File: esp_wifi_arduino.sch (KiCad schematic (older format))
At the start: 32 parts, among them IC1 ATMEGA328P-A, P1 CONN_01X15, P2 CONN_01X15, P5 CONN_01X04, P6 CONN_01X04, SW1 SW_PUSH, SW2 SW_PUSH, SW3 DIPSW4, U1 ADG3304, U2 ESP-WROOM-02, U3 NJM2391DL1-33, X1 16MHz

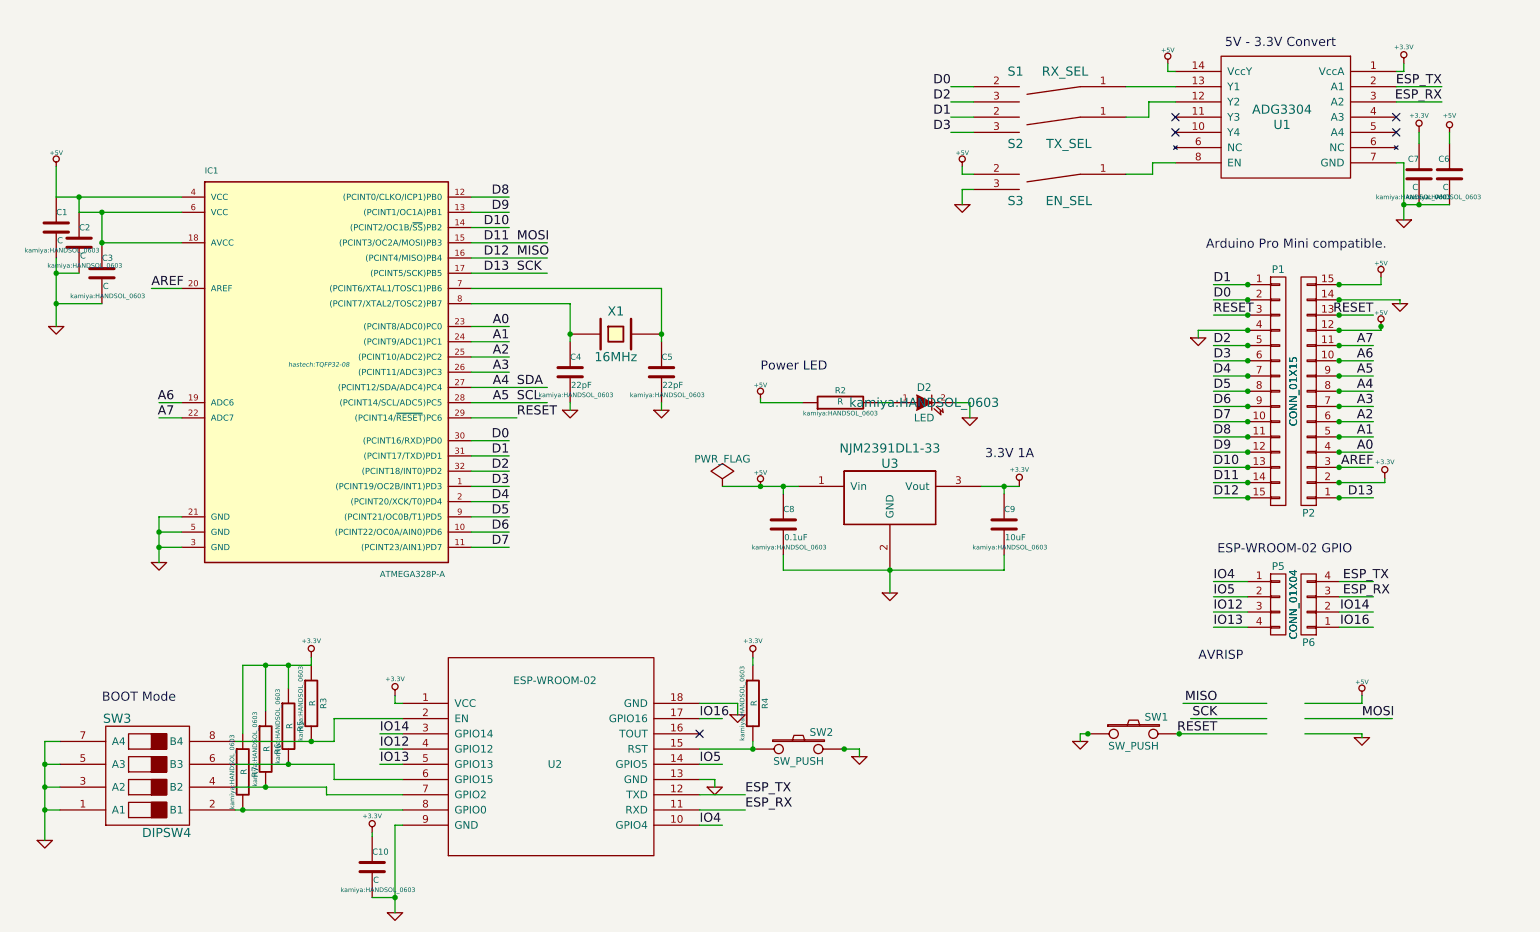
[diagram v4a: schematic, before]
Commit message: Draw Pattern
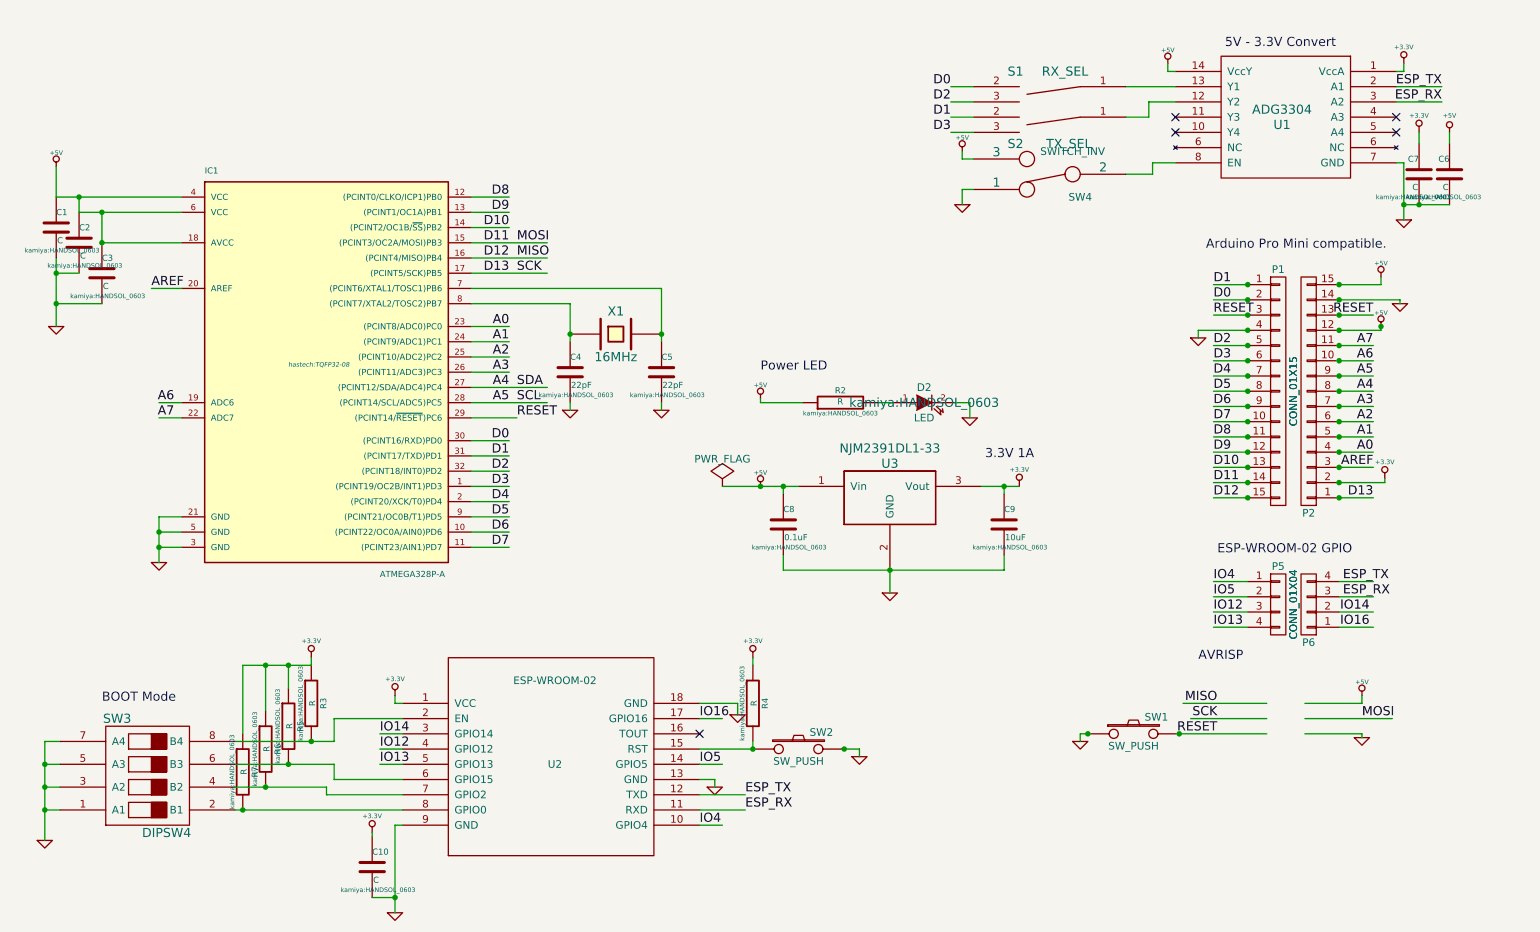
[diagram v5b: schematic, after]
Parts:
- removed S3: EN_SEL, kamiya:ALPS_SSSS213202(SlideSW), symbol SEL
- added SW4: SWITCH_INV, ~, symbol SWITCH_INV
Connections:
- wire segments 202 -> 178
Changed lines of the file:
@@
 $EndComp
 $Comp
-L GND-RESCUE-esp_wifi_arduino #PWR019
+L GND-RESCUE-esp_wifi_arduino #PWR018
 U 1 1 562B5CFD
 P 4525 3875
-F 0 "#PWR019" H 4525 3875 30  0001 C CNN
+F 0 "#PWR018" H 4525 3875 30  0001 C CNN
 F 1 "GND" H 4525 3805 30  0001 C CNN
 F 2 "" H 4525 3875 60  0000 C CNN
@@
 $EndComp
 $Comp
-L GND-RESCUE-esp_wifi_arduino #PWR020
+L GND-RESCUE-esp_wifi_arduino #PWR019
 U 1 1 562B5D6B
 P 5125 3875
-F 0 "#PWR020" H 5125 3875 30  0001 C CNN
+F 0 "#PWR019" H 5125 3875 30  0001 C CNN
 F 1 "GND" H 5125 3805 30  0001 C CNN
 F 2 "" H 5125 3875 60  0000 C CNN
@@
 RESET
 $Comp
-L +5V #PWR021
+L +5V #PWR020
 U 1 1 562B67E1
 P 9725 5750
-F 0 "#PWR021" H 9725 5840 20  0001 C CNN
+F 0 "#PWR020" H 9725 5840 20  0001 C CNN
 F 1 "+5V" H 9725 5840 30  0000 C CNN
 F 2 "" H 9725 5750 60  0000 C CNN
@@
 $EndComp
 $Comp
-L GND-RESCUE-esp_wifi_arduino #PWR022
+L GND-RESCUE-esp_wifi_arduino #PWR021
 U 1 1 562B67E7
 P 9725 6025
-F 0 "#PWR022" H 9725 6025 30  0001 C CNN
+F 0 "#PWR021" H 9725 6025 30  0001 C CNN
 F 1 "GND" H 9725 5955 30  0001 C CNN
 F 2 "" H 9725 6025 60  0000 C CNN
@@
 $EndComp
 $Comp
-L GND-RESCUE-esp_wifi_arduino #PWR023
+L GND-RESCUE-esp_wifi_arduino #PWR022
 U 1 1 562B6DA0
 P 7150 3925
-F 0 "#PWR023" H 7150 3925 30  0001 C CNN
+F 0 "#PWR022" H 7150 3925 30  0001 C CNN
 F 1 "GND" H 7150 3855 30  0001 C CNN
 F 2 "" H 7150 3925 60  0000 C CNN
@@
 $EndComp
 $Comp
-L +5V #PWR024
+L +5V #PWR023
 U 1 1 562B6DA9
 P 5775 3800
-F 0 "#PWR024" H 5775 3890 20  0001 C CNN
+F 0 "#PWR023" H 5775 3890 20  0001 C CNN
 F 1 "+5V" H 5775 3890 30  0000 C CNN
 F 2 "" H 5775 3800 60  0000 C CNN
@@
 $EndComp
 $Comp
-L GND-RESCUE-esp_wifi_arduino #PWR025
+L GND-RESCUE-esp_wifi_arduino #PWR024
 U 1 1 562B7055
 P 7875 6050
-F 0 "#PWR025" H 7875 6050 30  0001 C CNN
+F 0 "#PWR024" H 7875 6050 30  0001 C CNN
 F 1 "GND" H 7875 5980 30  0001 C CNN
 F 2 "" H 7875 6050 60  0000 C CNN
@@
 D12
 $Comp
-L GND-RESCUE-esp_wifi_arduino #PWR026
+L GND-RESCUE-esp_wifi_arduino #PWR025
 U 1 1 562B7319
 P 8650 3400
-F 0 "#PWR026" H 8650 3400 30  0001 C CNN
+F 0 "#PWR025" H 8650 3400 30  0001 C CNN
 F 1 "GND" H 8650 3330 30  0001 C CNN
 F 2 "" H 8650 3400 60  0000 C CNN
@@
 A0
 $Comp
-L +3.3V-RESCUE-esp_wifi_arduino #PWR027
+L +3.3V-RESCUE-esp_wifi_arduino #PWR026
 U 1 1 562B76DE
 P 9875 4325
-F 0 "#PWR027" H 9875 4285 30  0001 C CNN
+F 0 "#PWR026" H 9875 4285 30  0001 C CNN
 F 1 "+3.3V" H 9875 4435 30  0000 C CNN
 F 2 "" H 9875 4325 60  0000 C CNN
@@
 $EndComp
 $Comp
-L +5V #PWR028
+L +5V #PWR027
 U 1 1 562B76E4
 P 9850 3000
-F 0 "#PWR028" H 9850 3090 20  0001 C CNN
+F 0 "#PWR027" H 9850 3090 20  0001 C CNN
 F 1 "+5V" H 9850 3090 30  0000 C CNN
 F 2 "" H 9850 3000 60  0000 C CNN
@@
 $EndComp
 $Comp
-L +5V #PWR029
+L +5V #PWR028
 U 1 1 562B76EA
 P 9850 3325
-F 0 "#PWR029" H 9850 3415 20  0001 C CNN
+F 0 "#PWR028" H 9850 3415 20  0001 C CNN
 F 1 "+5V" H 9850 3415 30  0000 C CNN
 F 2 "" H 9850 3325 60  0000 C CNN
@@
 $EndComp
 $Comp
-L GND-RESCUE-esp_wifi_arduino #PWR030
+L GND-RESCUE-esp_wifi_arduino #PWR029
 U 1 1 562B76F0
 P 9975 3175
-F 0 "#PWR030" H 9975 3175 30  0001 C CNN
+F 0 "#PWR029" H 9975 3175 30  0001 C CNN
 F 1 "GND" H 9975 3105 30  0001 C CNN
 F 2 "" H 9975 3175 60  0000 C CNN
@@
 $EndComp
 $Comp
-L +5V #PWR031
+L +5V #PWR030
 U 1 1 562B7AC7
 P 10300 2050
-F 0 "#PWR031" H 10300 2140 20  0001 C CNN
+F 0 "#PWR030" H 10300 2140 20  0001 C CNN
 F 1 "+5V" H 10300 2160 30  0000 C CNN
 F 2 "" H 10300 2050 60  0000 C CNN
@@
 $EndComp
 $Comp
-L +3.3V-RESCUE-esp_wifi_arduino #PWR032
+L +3.3V-RESCUE-esp_wifi_arduino #PWR031
 U 1 1 562B7C34
 P 10100 2050
-F 0 "#PWR032" H 10100 2010 30  0001 C CNN
+F 0 "#PWR031" H 10100 2010 30  0001 C CNN
 F 1 "+3.3V" H 10100 2160 30  0000 C CNN
 F 2 "" H 10100 2050 60  0000 C CNN
@@
 $EndComp
 $Comp
-L +3.3V-RESCUE-esp_wifi_arduino #PWR033
+L +3.3V-RESCUE-esp_wifi_arduino #PWR032
 U 1 1 562B81D7
 P 3225 6650
-F 0 "#PWR033" H 3225 6610 30  0001 C CNN
+F 0 "#PWR032" H 3225 6610 30  0001 C CNN
 F 1 "+3.3V" H 3225 6760 30  0000 C CNN
 F 2 "" H 3225 6650 60  0000 C CNN
@@
 $EndComp
 $Comp
-L SEL S3
-U 1 1 565B9EEA
-P 7725 2325
-F 0 "S3" H 8000 2500 60  0000 C CNN
-F 1 "EN_SEL" H 7650 2500 60  0000 C CNN
-F 2 "kamiya:ALPS_SSSS213202(SlideSW)" H 7725 2325 60  0001 C CNN
-F 3 "" H 7725 2325 60  0000 C CNN
-	1    7725 2325
-	-1   0    0    1
-$EndComp
-$Comp
-L +5V #PWR034
+L +5V #PWR033
 U 1 1 565BAAFD
-P 7100 2275
-F 0 "#PWR034" H 7100 2365 20  0001 C CNN
-F 1 "+5V" H 7100 2365 30  0000 C CNN
-F 2 "" H 7100 2275 60  0000 C CNN
-F 3 "" H 7100 2275 60  0000 C CNN
-	1    7100 2275
+P 7100 2175
+F 0 "#PWR033" H 7100 2265 20  0001 C CNN
+F 1 "+5V" H 7100 2265 30  0000 C CNN
+F 2 "" H 7100 2175 60  0000 C CNN
+F 3 "" H 7100 2175 60  0000 C CNN
+	1    7100 2175
 	-1   0    0    -1
 $EndComp
 $Comp
-L GND-RESCUE-esp_wifi_arduino #PWR035
+L GND-RESCUE-esp_wifi_arduino #PWR034
 U 1 1 565BB608
 P 7100 2525
-F 0 "#PWR035" H 7100 2525 30  0001 C CNN
+F 0 "#PWR034" H 7100 2525 30  0001 C CNN
 F 1 "GND" H 7100 2455 30  0001 C CNN
 F 2 "" H 7100 2525 60  0000 C CNN
@@
 $EndComp
 Wire Wire Line
-	5525 4375 5775 4375
-Wire Wire Line
-	5775 4375 5925 4375
-Wire Wire Line
-	5925 4375 6025 4375
+	5525 4375 6025 4375
 Wire Wire Line
 	5925 4425 5925 4375
@@
 	5925 4825 5925 4925
 Wire Wire Line
-	5925 4925 6625 4925
-Wire Wire Line
-	6625 4925 7375 4925
+	5925 4925 7375 4925
 Wire Wire Line
 	7375 4925 7375 4825
 Connection ~ 6625 4925
 Wire Wire Line
-	7225 4375 7375 4375
-Wire Wire Line
-	7375 4375 7475 4375
+	7225 4375 7475 4375
 Wire Wire Line
 	7375 4375 7375 4425
@@
 	9950 2250 10000 2250
 Wire Wire Line
-	10000 2250 10000 2525
-Wire Wire Line
-	10000 2525 10000 2625
+	10000 2250 10000 2625
 Wire Wire Line
 	9950 1750 10250 1750
@@
 	1150 2275 1150 2475
 Wire Wire Line
-	1150 2475 1300 2475
-Wire Wire Line
-	1300 2475 1975 2475
-Wire Wire Line
-	1300 2575 1450 2575
-Wire Wire Line
-	1450 2575 1975 2575
+	1150 2475 1975 2475
+Wire Wire Line
+	1300 2575 1975 2575
 Wire Wire Line
 	1300 2575 1300 2475
@@
 	1300 2975 1150 2975
 Wire Wire Line
-	1150 2875 1150 2975
-Wire Wire Line
-	1150 2975 1150 3175
-Wire Wire Line
-	1150 3175 1150 3325
+	1150 2875 1150 3325
 Connection ~ 1150 2975
 Wire Wire Line
@@
 	1975 4575 1825 4575
 Wire Wire Line
-	1825 4575 1825 4675
-Wire Wire Line
-	1825 4675 1825 4775
-Wire Wire Line
-	1825 4775 1825 4875
+	1825 4575 1825 4875
 Wire Wire Line
 	1975 4675 1825 4675
@@
 	3425 6600 3375 6600
 Wire Wire Line
-	3375 6600 3375 7075
-Wire Wire Line
-	3375 7075 3375 7175
+	3375 6600 3375 7175
 Wire Wire Line
 	5375 6300 5475 6300
@@
 	5475 6300 5475 6350
 Wire Wire Line
-	2325 6500 2375 6500
-Wire Wire Line
-	2375 6500 3425 6500
+	2325 6500 3425 6500
 Wire Wire Line
 	3425 6400 2925 6400
@@
 	2925 6400 2925 6350
 Wire Wire Line
-	2925 6350 2525 6350
-Wire Wire Line
-	2525 6350 2325 6350
+	2925 6350 2325 6350
 Wire Wire Line
 	3425 6300 2975 6300
@@
 	2975 6300 2975 6200
 Wire Wire Line
-	2975 6200 2675 6200
-Wire Wire Line
-	2675 6200 2325 6200
+	2975 6200 2325 6200
 Wire Wire Line
 	3425 5900 2975 5900
@@
 	2975 5900 2975 6050
 Wire Wire Line
-	2975 6050 2825 6050
-Wire Wire Line
-	2825 6050 2325 6050
+	2975 6050 2325 6050
 Wire Wire Line
 	3375 5750 3375 5800
@@
 	2825 5550 2825 5500
 Wire Wire Line
-	2375 5550 2525 5550
-Wire Wire Line
-	2525 5550 2675 5550
-Wire Wire Line
-	2675 5550 2825 5550
+	2375 5550 2825 5550
 Wire Wire Line
 	2675 5550 2675 5700
@@
 	1075 6500 1175 6500
 Wire Wire Line
-	1075 6050 1075 6200
-Wire Wire Line
-	1075 6200 1075 6350
-Wire Wire Line
-	1075 6350 1075 6500
-Wire Wire Line
-	1075 6500 1075 6700
+	1075 6050 1075 6700
 Wire Wire Line
 	1175 6350 1075 6350
@@
 	5125 3825 5125 3875
 Wire Wire Line
-	5125 3075 5125 3375
-Wire Wire Line
-	5125 3375 5125 3425
-Wire Wire Line
-	4525 3175 4525 3375
-Wire Wire Line
-	4525 3375 4525 3425
+	5125 3075 5125 3425
+Wire Wire Line
+	4525 3175 4525 3425
 Wire Wire Line
 	4525 3175 3875 3175
@@
 	9875 4350 9875 4325
 Wire Wire Line
-	10000 2525 10100 2525
-Wire Wire Line
-	10100 2525 10300 2525
+	10000 2525 10300 2525
 Connection ~ 10000 2525
 Wire Wire Line
@@
 	8325 1950 8175 1950
 Wire Wire Line
-	7100 2275 7100 2325
-Wire Wire Line
-	7100 2325 7175 2325
+	7100 2175 7100 2225
+Wire Wire Line
+	7100 2225 7175 2225
 Wire Wire Line
 	7175 2425 7100 2425
@@
 NoConn ~ 9950 2050
 $Comp
-L PWR_FLAG #FLG036
+L PWR_FLAG #FLG035
 U 1 1 565D8F5F
 P 5525 4375
-F 0 "#FLG036" H 5525 4470 50  0001 C CNN
+F 0 "#FLG035" H 5525 4470 50  0001 C CNN
 F 1 "PWR_FLAG" H 5525 4555 50  0000 C CNN
 F 2 "" H 5525 4375 60  0000 C CNN
@@
 Connection ~ 5775 4375
 NoConn ~ 5375 6000
+$Comp
+L SWITCH_INV SW4
+U 1 1 565B1479
+P 7675 2325
+F 0 "SW4" H 7475 2475 50  0000 C CNN
+F 1 "SWITCH_INV" H 7525 2175 50  0000 C CNN
+F 2 "~" H 7675 2325 60  0000 C CNN
+F 3 "~" H 7675 2325 60  0000 C CNN
+	1    7675 2325
+	-1   0    0    1
+$EndComp
 $EndSCHEMATC

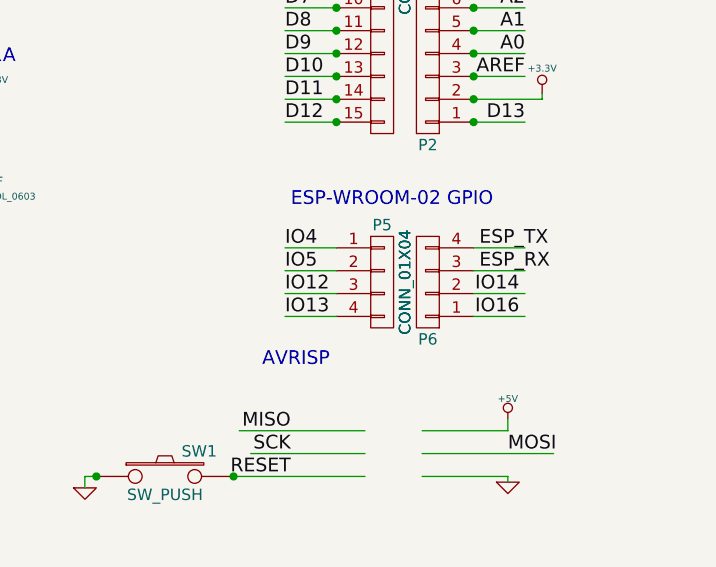
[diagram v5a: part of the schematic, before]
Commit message: Create Production File
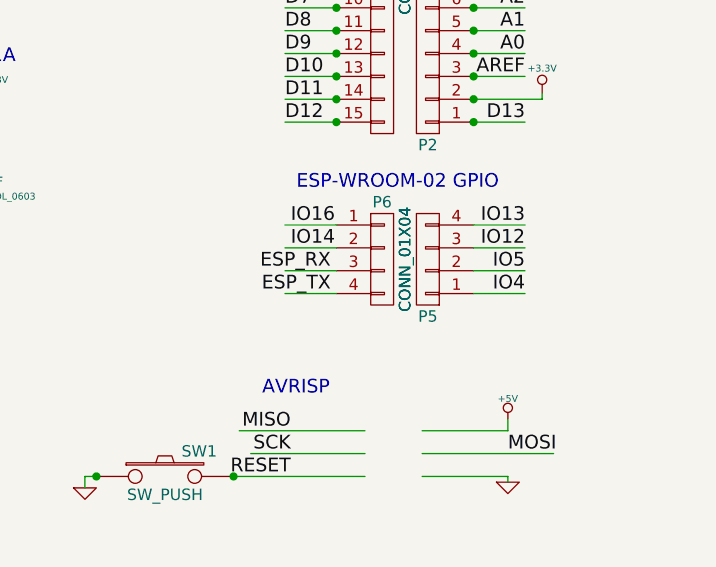
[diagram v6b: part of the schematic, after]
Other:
- moved on the sheet: P5, P6
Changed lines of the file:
@@
 Sheet 1 1
 Title "Arduino with ESP-WROOM-02"
-Date "29 nov 2015"
+Date "30 nov 2015"
 Rev "A"
 Comp "Asumono-LAB"
@@
 Text Notes 1450 5800 0    60   ~ 0
 BOOT Mode
-Text Notes 8650 5525 0    60   ~ 0
+Text Notes 8650 5650 0    60   ~ 0
 AVRISP
 Text Label 7025 1750 2    60   ~ 0
@@
 	8350 2325 8175 2325
 Wire Wire Line
+	9575 5200 9800 5200
+Wire Wire Line
+	9575 5100 9800 5100
+Wire Wire Line
+	9575 5000 9800 5000
+Wire Wire Line
+	8975 5200 8750 5200
+Wire Wire Line
+	8975 5100 8750 5100
+Wire Wire Line
 	8975 5000 8750 5000
-Wire Wire Line
-	8975 5100 8750 5100
-Wire Wire Line
-	8975 5200 8750 5200
-Wire Wire Line
-	9575 5000 9800 5000
-Wire Wire Line
-	9575 5100 9800 5100
-Wire Wire Line
-	9575 5200 9800 5200
 Wire Wire Line
 	5625 5800 5625 5875
@@
 Text Label 3275 6200 0    60   ~ 0
 IO13
-Text Label 9775 5200 2    60   ~ 0
+Text Label 8775 5000 0    60   ~ 0
 IO14
-Text Label 8750 5200 0    60   ~ 0
+Text Label 9800 5000 2    60   ~ 0
 IO12
-Text Label 8750 5300 0    60   ~ 0
+Text Label 9800 4900 2    60   ~ 0
 IO13
-Text Label 8750 5000 0    60   ~ 0
+Text Label 9800 5200 2    60   ~ 0
 IO4
-Text Label 8750 5100 0    60   ~ 0
+Text Label 9800 5100 2    60   ~ 0
 IO5
-Text Label 9775 5300 2    60   ~ 0
+Text Label 8775 4900 0    60   ~ 0
 IO16
 $Comp
 L CONN_01X04 P5
 U 1 1 565CD625
-P 9175 5150
-F 0 "P5" H 9175 5400 50  0000 C CNN
-F 1 "CONN_01X04" V 9275 5150 50  0000 C CNN
-F 2 "Pin_Headers:Pin_Header_Straight_1x04" H 9175 5150 60  0001 C CNN
-F 3 "" H 9175 5150 60  0000 C CNN
-	1    9175 5150
-	1    0    0    -1
+P 9375 5050
+F 0 "P5" H 9375 5300 50  0000 C CNN
+F 1 "CONN_01X04" V 9475 5050 50  0000 C CNN
+F 2 "Pin_Headers:Pin_Header_Straight_1x04" H 9375 5050 60  0001 C CNN
+F 3 "" H 9375 5050 60  0000 C CNN
+	1    9375 5050
+	-1   0    0    1
 $EndComp
 $Comp
 L CONN_01X04 P6
 U 1 1 565CD6C2
-P 9375 5150
-F 0 "P6" H 9375 5400 50  0000 C CNN
-F 1 "CONN_01X04" V 9475 5150 50  0000 C CNN
-F 2 "Pin_Headers:Pin_Header_Straight_1x04" H 9375 5150 60  0001 C CNN
-F 3 "" H 9375 5150 60  0000 C CNN
-	1    9375 5150
-	-1   0    0    1
-$EndComp
-Wire Wire Line
-	8975 5300 8750 5300
-Wire Wire Line
-	9575 5300 9800 5300
-Text Notes 8775 4825 0    60   ~ 0
+P 9175 5050
+F 0 "P6" H 9175 5300 50  0000 C CNN
+F 1 "CONN_01X04" V 9275 5050 50  0000 C CNN
+F 2 "Pin_Headers:Pin_Header_Straight_1x04" H 9175 5050 60  0001 C CNN
+F 3 "" H 9175 5050 60  0000 C CNN
+	1    9175 5050
+	1    0    0    -1
+$EndComp
+Wire Wire Line
+	9575 4900 9800 4900
+Wire Wire Line
+	8975 4900 8750 4900
+Text Notes 8800 4750 0    60   ~ 0
 ESP-WROOM-02 GPIO
 Text Label 10250 1750 2    60   ~ 0
@@
 Text Label 10250 1850 2    60   ~ 0
 ESP_RX
-Text Label 9600 5000 0    60   ~ 0
+Text Label 8950 5200 2    60   ~ 0
 ESP_TX
-Text Label 9600 5100 0    60   ~ 0
+Text Label 8950 5100 2    60   ~ 0
 ESP_RX
 NoConn ~ 8500 1950
